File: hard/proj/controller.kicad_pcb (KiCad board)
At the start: 2 copper layers, 44 parts, among them J1 microUSB, J2 EXT1, J3 EXT2, J4 EXT3, J5 EXT4, J6 UART, Q1 BC848B, Q2 BC848B, Q3 BC848B, Q4 BC848B, SW1 RESET, SW2 FLASH, U1 LM3940, U2 ESP-07v2

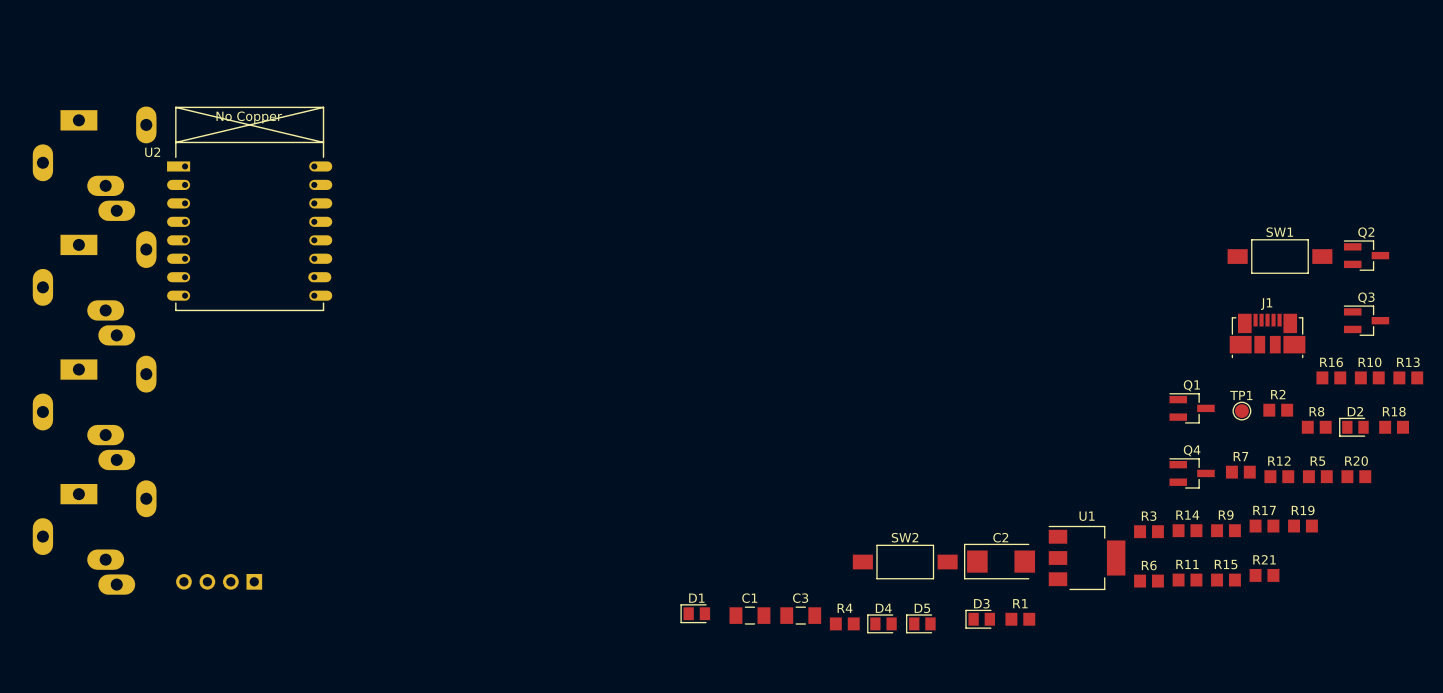
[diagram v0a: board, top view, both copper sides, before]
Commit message: layouted
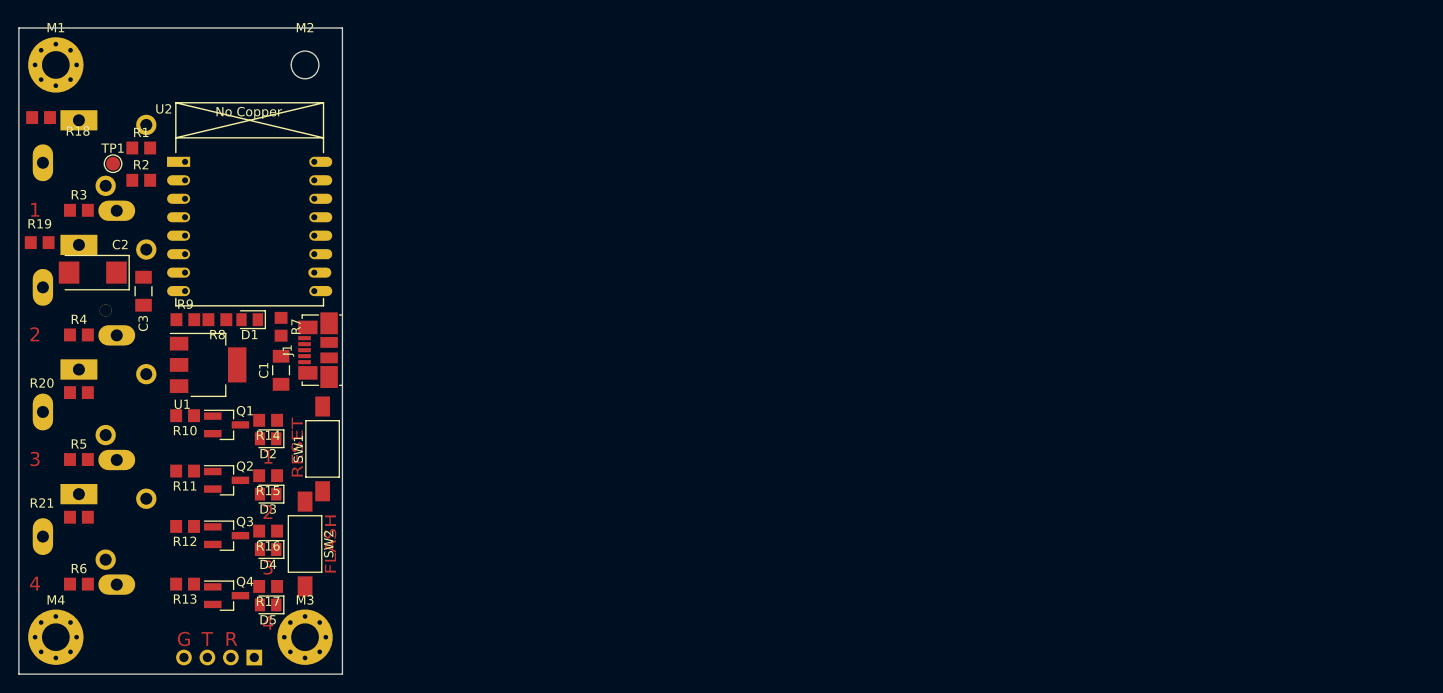
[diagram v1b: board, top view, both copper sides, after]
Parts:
- added M1: MountingHole_3mm_Pad_Via, MountingHole:MountingHole_3mm_Pad_Via, F.Cu at (36.0, 92.5)
- added M2: MountingHole_3mm, MountingHole:MountingHole_3mm, F.Cu at (63.0, 92.5)
- added M3: MountingHole_3mm_Pad_Via, MountingHole:MountingHole_3mm_Pad_Via, F.Cu at (63.0, 154.5)
- added M4: MountingHole_3mm_Pad_Via, MountingHole:MountingHole_3mm_Pad_Via, F.Cu at (36.0, 154.5)
- moved R18 150.4 mm to (34.4, 98.2), turned to 180 degrees
- moved R19 140.3 mm to (34.2, 111.8), turned to 180 degrees
- moved R20 138.7 mm to (38.5, 128.0)
- moved R13 134.4 mm to (50.0, 148.8), turned to 180 degrees
- moved R5 134.2 mm to (38.5, 135.2)
- moved R21 128.6 mm to (38.5, 141.5)
- moved R10 128.4 mm to (50.0, 130.5), turned to 180 degrees
- moved Q2 125.9 mm to (54.5, 137.5)
- moved Q3 125.7 mm to (54.5, 143.5)
- moved R2 125.7 mm to (45.2, 105.0)
- moved TP1 125.2 mm to (42.2, 103.2)
- moved R3 121.1 mm to (38.5, 108.2)
- moved R8 119.7 mm to (53.5, 120.1), turned to 180 degrees
- moved R12 118.7 mm to (50.0, 142.5), turned to 180 degrees
- moved D2 117.8 mm to (59.0, 133.0), turned to 180 degrees
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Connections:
- J1 pad 6: Net-(J1-Pad6) -> (no net)
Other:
- board outline added: 35 x 70 mm
- board text added: "1"
- board text added: "2"
- board text added: "3"
- board text added: "4"
- board text added: "FLASH"
- board text added: "G"
- board text added: "R"
- board text added: "RESET"
- board text added: "T"

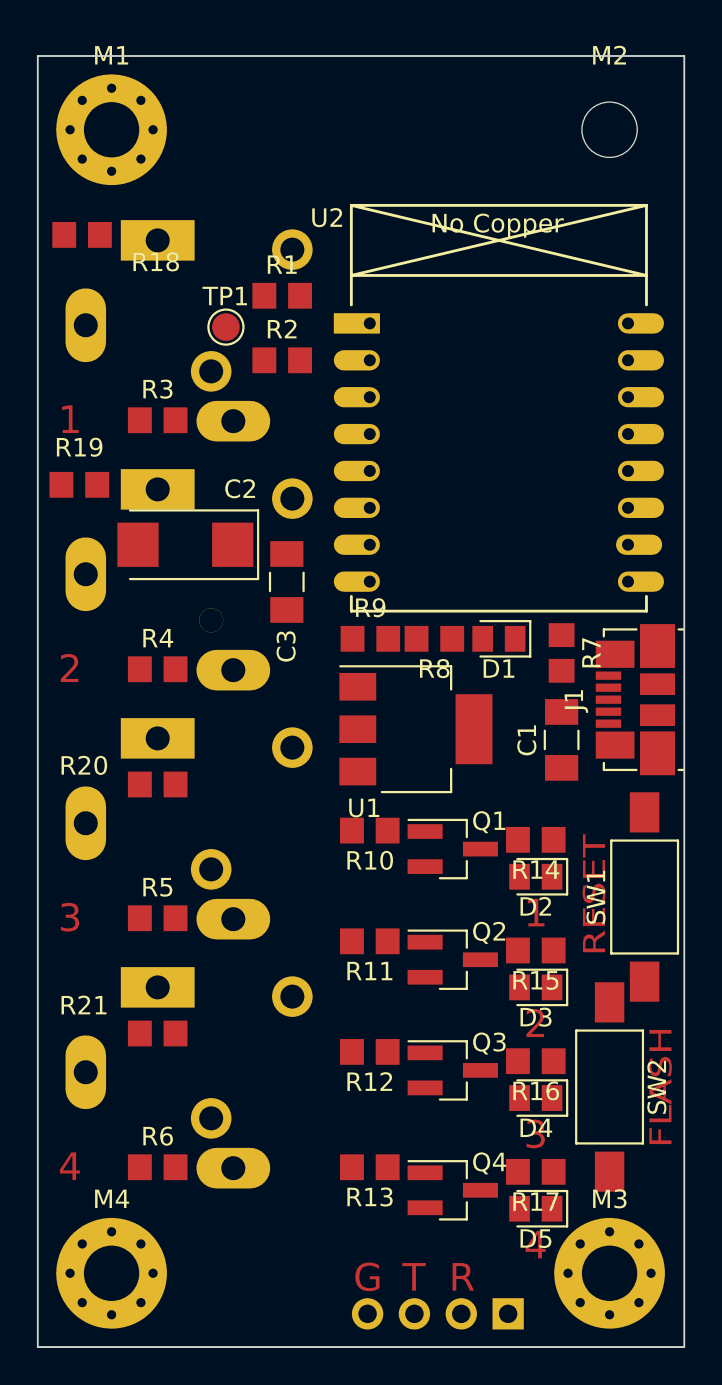
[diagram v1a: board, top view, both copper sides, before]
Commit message: routing
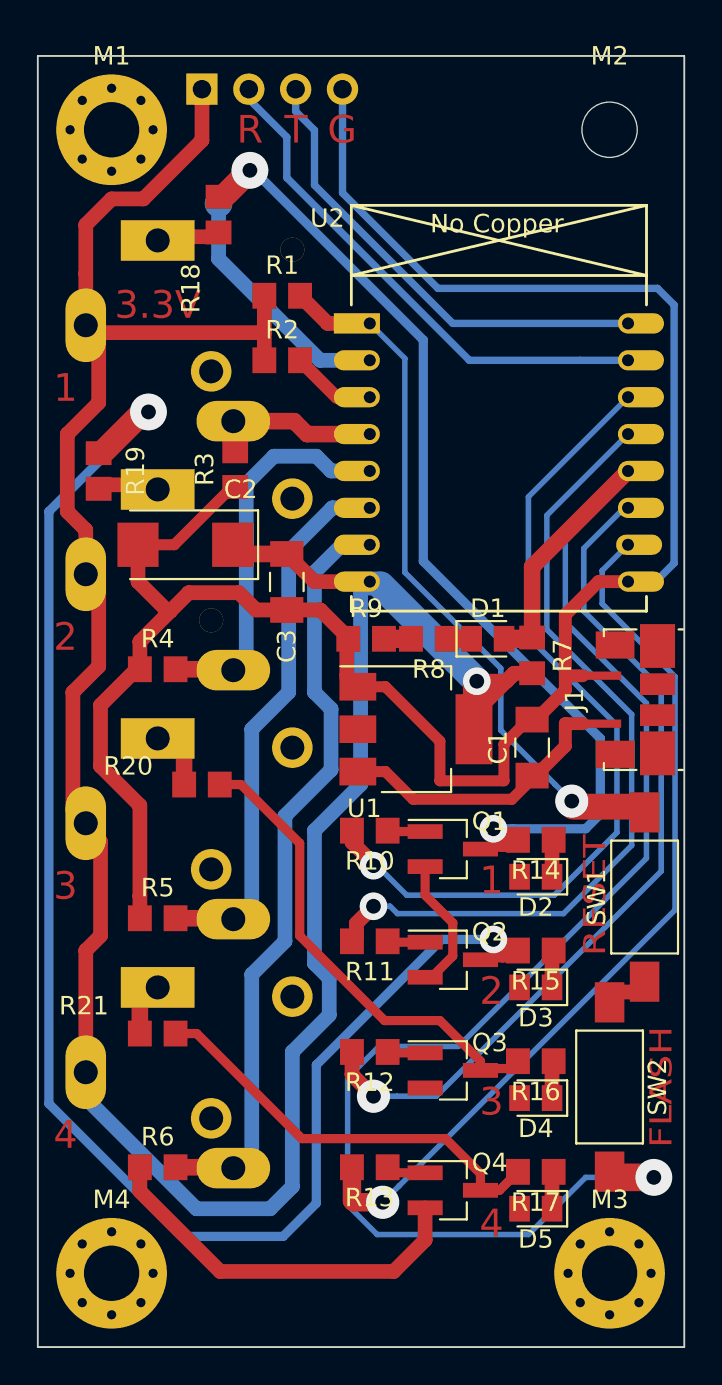
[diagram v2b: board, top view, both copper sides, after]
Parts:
- TP1: moved to B.Cu
- moved J6 68.4 mm to (40.9, 90.3), turned to 270 degrees
- moved R18 7.48 mm to (41.8, 97.1), turned to 90 degrees
- moved TP1 6.71 mm to (41.8, 96.5)
- moved R3 4.97 mm to (42.7, 110.9), turned to 90 degrees
- moved R20 2.40 mm to (40.9, 128.0)
- moved C1 1.65 mm to (58.8, 126.0)
- moved R7 1.61 mm to (58.8, 121.0)
- moved R19 1.29 mm to (35.3, 111.0), turned to 90 degrees
- moved D1 0.60 mm to (56.4, 120.1), turned to 0 degrees
- moved R8 0.30 mm to (53.2, 120.1)
- moved R9 0.23 mm to (49.8, 120.1)
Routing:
- net +3V3: track 0.00 -> 149.6 mm, vias 0 -> 1
- net GND: track 0.00 -> 144.2 mm
- net /FLASH: track 0.00 -> 85.2 mm, vias 0 -> 1
- net /LED2_PWR: track 0.00 -> 84.5 mm, vias 0 -> 2
- net /LED1_PWR: track 0.00 -> 53.9 mm, vias 0 -> 2
- net /LED4_CTL: track 0.00 -> 48.2 mm, vias 0 -> 1
- net /LED3_CTL: track 0.00 -> 46.1 mm, vias 0 -> 1
- net /LED1_CTL: track 0.00 -> 45.5 mm, vias 0 -> 1
- net /LED2_CTL: track 0.00 -> 44.1 mm, vias 0 -> 1
- net /BTN4: track 0.00 -> 41.1 mm
- net /RESET: track 0.00 -> 38.5 mm, vias 0 -> 1
- net /BTN3: track 0.00 -> 29.2 mm
- net /PC_TX: track 0.00 -> 28.3 mm
- net /PC_RX: track 0.00 -> 25.7 mm
- net /LED3_PWR: track 0.00 -> 25.3 mm
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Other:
- net class Default: clearance 0.2 -> 0.3; trace_width 0.25 -> 0.4; via_dia 0.8 -> 1; via_drill 0.4 -> 0.8
- net class Power added: clearance 0.3, trace_width 0.6, via_dia 1, via_drill 0.8
- net class Signal added: clearance 0.3, trace_width 0.3, via_dia 1, via_drill 0.8
- rule trace_clearance: 0.2 -> 0.3
- rule trace_min: 0.2 -> 0.3
- rule via_min_drill: 0.3 -> 0.8
- rule via_min_size: 0.4 -> 0.8
- board text added: "3.3V"
